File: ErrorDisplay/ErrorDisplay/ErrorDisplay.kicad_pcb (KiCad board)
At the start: 2 copper layers, 204.2 x 62.3 mm, 7 parts, among them J1 X27Motor, J2 X27Motor, J3 X27Motor

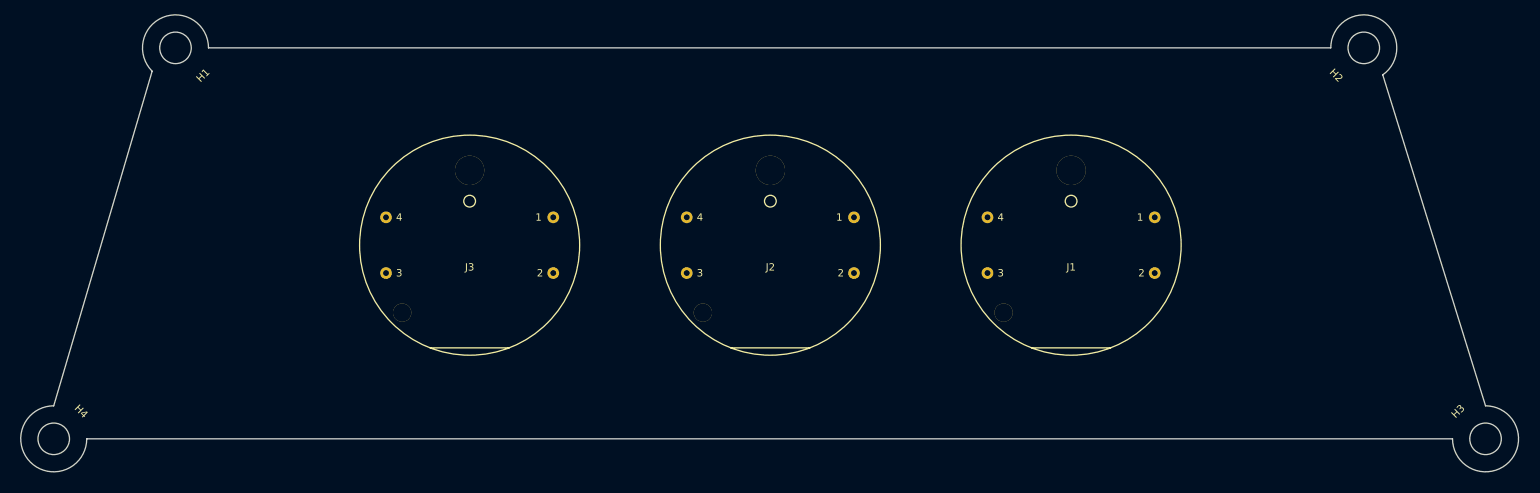
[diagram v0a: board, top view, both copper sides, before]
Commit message: WIP - Test build for the Stepper Driver
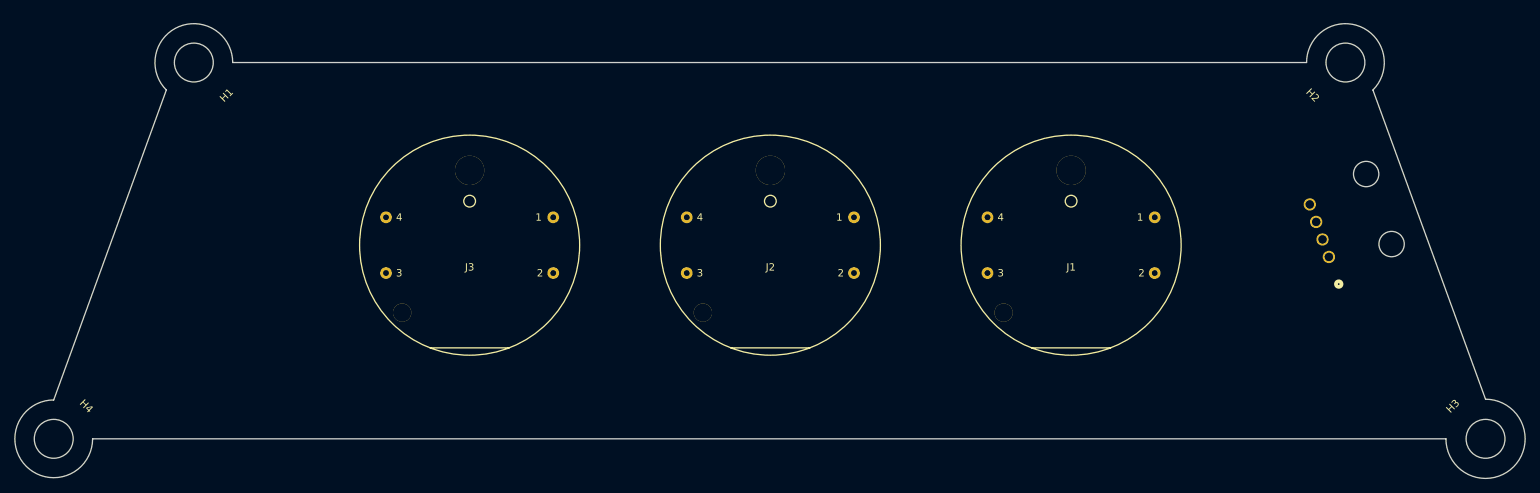
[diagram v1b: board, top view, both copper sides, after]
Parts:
- added J4: Conn_01x04_Pin, Library:CONN_70551-xxxx_04_MOL, B.Cu at (221.2, 110.9)
- H1, H2, H3, H4: footprint MountingHole:MountingHole_4.3mm_M4 -> MountingHole:MountingHole_5.3mm_M5
- moved H1 3.20 mm to (66.5, 84.4)
- moved H2 3.20 mm to (223.5, 84.4)
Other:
- board size 204.2 x 62.3 mm -> 205.9 x 62 mm
